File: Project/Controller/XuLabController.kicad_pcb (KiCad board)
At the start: 4 copper layers, 115 x 123 mm, 75 parts, among them J1 SWD Connector, J10 Servo, J11 Servo, J12 Thruster, J13 USB_B_Micro, J14 CAN, J15 I2C, J16 UART, J2 Conn_01x04, J3 1986660-2, J4 Servo, J5 Servo, J6 Servo, J7 Servo, J8 Servo, J9 Servo, Q2 PMOS, SW1 SW_Push, SW2 SW_SPDT, SW3 SW_SPDT, U1 STM32F446RCTx, U2 BMI088, U3 MMC5983MA, U4 AP63203WU, U5 TVS0500DRV, Y1 25 MHz

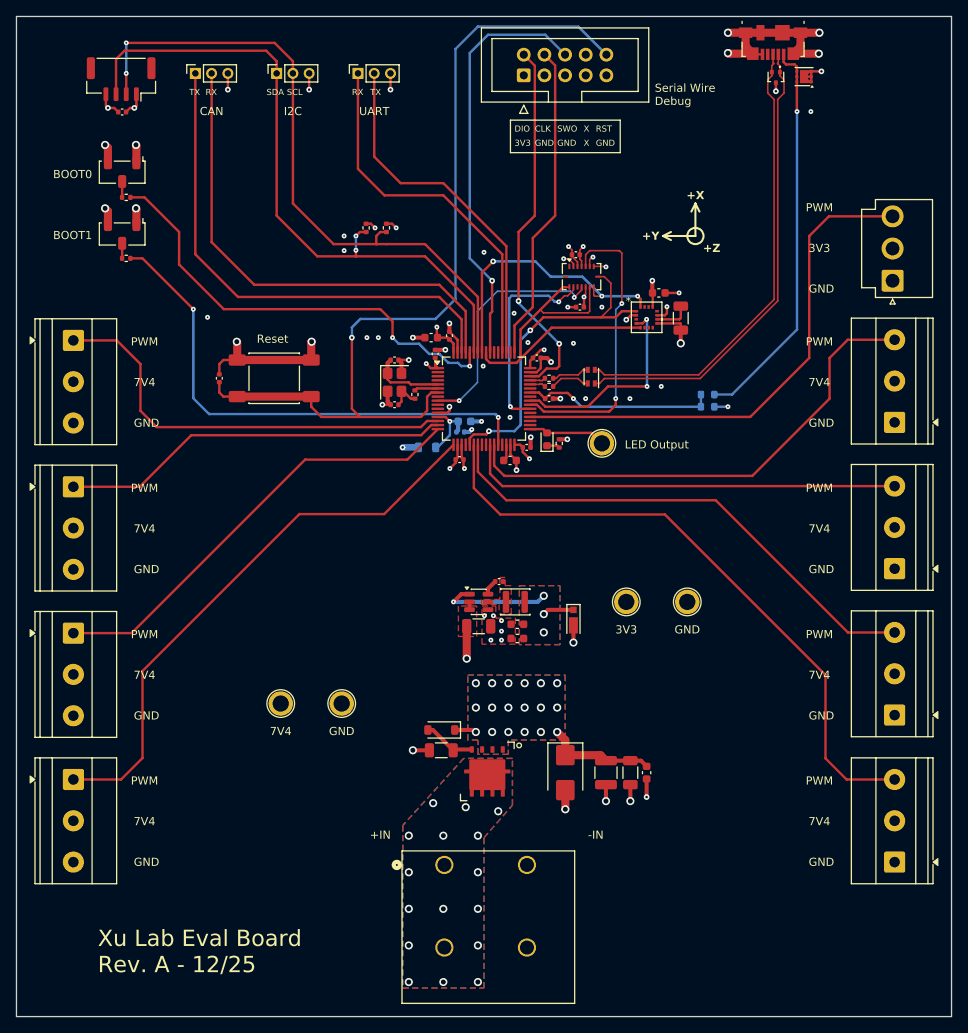
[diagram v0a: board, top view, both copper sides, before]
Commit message: Add initial layout
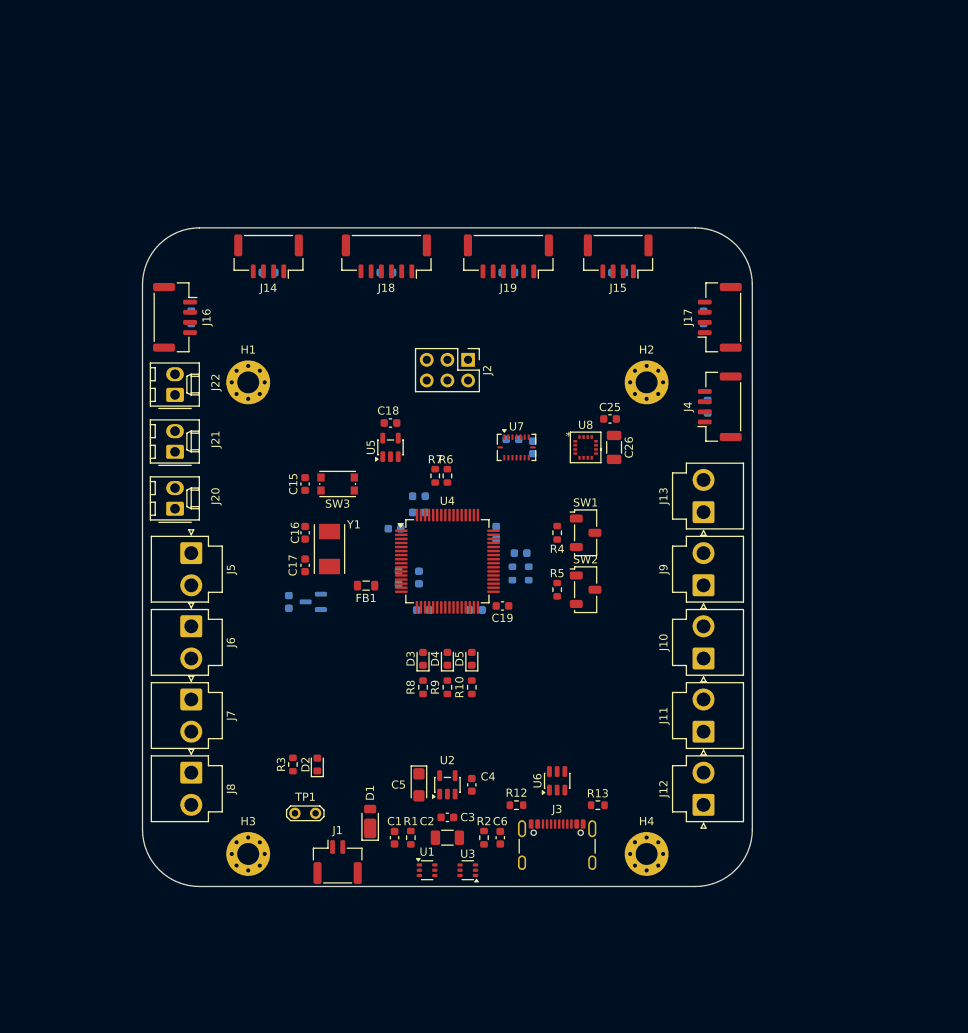
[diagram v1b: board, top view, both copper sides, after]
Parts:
- removed FL1: 0805USB-502MLC, Inductor_SMD:L_CommonModeChoke_Coilcraft_0805USB
- removed L1: 3.9uH, Inductor_SMD:L_Pulse_PA4334
- removed Q2: PMOS, XuLab:SOP-Advance-8
- removed TP2, TP3, TP4, TP5: TestPoint, TestPoint:TestPoint_Plated_Hole_D2.0mm
- added C26: 10uF, Capacitor_SMD:C_1206_3216Metric, F.Cu at (166.0, 86.0)
- added C27: 100nF, Capacitor_SMD:C_0603_1608Metric, B.Cu at (123.5, 64.5)
- added C28: 100nF, Capacitor_SMD:C_0603_1608Metric, B.Cu at (166.5, 64.5)
- added C29: 100nF, Capacitor_SMD:C_0603_1608Metric, B.Cu at (114.0, 70.0)
- added C30: 100nF, Capacitor_SMD:C_0603_1608Metric, B.Cu at (177.0, 70.0)
- added C31: 100nF, Capacitor_SMD:C_0603_1608Metric, B.Cu at (138.0, 64.5)
- added C32: 100nF, Capacitor_SMD:C_0603_1608Metric, B.Cu at (153.0, 64.5)
- added H1: MH, MountingHole:MountingHole_2.7mm_M2.5_Pad_Via, F.Cu at (121.0, 78.0)
- added H2: MH, MountingHole:MountingHole_2.7mm_M2.5_Pad_Via, F.Cu at (170.0, 78.0)
- added H3: MH, MountingHole:MountingHole_2.7mm_M2.5_Pad_Via, F.Cu at (121.0, 136.0)
- added H4: MH, MountingHole:MountingHole_2.7mm_M2.5_Pad_Via, F.Cu at (170.0, 136.0)
- added J17: UART2, Connector_JST:JST_GH_SM04B-GHS-TB_1x04-1MP_P1.25mm_Horizontal, F.Cu at (179.0, 70.0)
- added J18: SPI1, Connector_JST:JST_GH_SM06B-GHS-TB_1x06-1MP_P1.25mm_Horizontal, F.Cu at (138.0, 62.5)
- added J19: SPI2, Connector_JST:JST_GH_SM06B-GHS-TB_1x06-1MP_P1.25mm_Horizontal, F.Cu at (153.0, 62.5)
- added J20: Interrupt, Connector_Molex:Molex_KK-254_AE-6410-02A_1x02_P2.54mm_Vertical, F.Cu at (112.0, 93.5)
- added J21: Interrupt, Connector_Molex:Molex_KK-254_AE-6410-02A_1x02_P2.54mm_Vertical, F.Cu at (112.0, 86.5)
- added J22: Interrupt, Connector_Molex:Molex_KK-254_AE-6410-02A_1x02_P2.54mm_Vertical, F.Cu at (112.0, 79.5)
- added R12: 5k1, Resistor_SMD:R_0603_1608Metric, F.Cu at (154.0, 130.0)
- added R13: 5k1, Resistor_SMD:R_0603_1608Metric, F.Cu at (164.0, 130.0)
- added R14: 82k, Resistor_SMD:R_0603_1608Metric, B.Cu at (155.5, 101.5)
- added U6: USBLC6-2SC6, Package_TO_SOT_SMD:SOT-23-6, F.Cu at (159.0, 127.0)
- added U7: BMI088, Package_LGA:Bosch_LGA-16_4.5x3mm_P0.5mm_LayoutBorder7x1y_ClockwisePinNumbering, F.Cu at (154.0, 86.0)
- added U8: MMC5983MA, XuLab:MMC5983MA_MEM, F.Cu at (162.5, 86.0)
- added U9: MCP9700Ax-ETT, Package_TO_SOT_SMD:SOT-23, B.Cu at (129.0, 105.0)
- C1: value 4.7uF -> 1uF
- C10, C14, C22: footprint Capacitor_SMD:C_0402_1005Metric -> Capacitor_SMD:C_0603_1608Metric; moved to B.Cu
- C11, C12: value 22pF -> 100nF; footprint Capacitor_SMD:C_0402_1005Metric -> Capacitor_SMD:C_0603_1608Metric; moved to B.Cu
- C13: value 100nF -> 1uF; footprint Capacitor_SMD:C_0402_1005Metric -> Capacitor_SMD:C_0603_1608Metric; moved to B.Cu
- C15: value 1uF -> 100nF
- C16: value 10uF -> 27pF; footprint Capacitor_SMD:C_1206_3216Metric -> Capacitor_SMD:C_0603_1608Metric
- C17: value 100nF -> 27pF; footprint Capacitor_SMD:C_0402_1005Metric -> Capacitor_SMD:C_0603_1608Metric
- C18: value 100uF -> 100nF; footprint Capacitor_SMD:C_1210_3225Metric -> Capacitor_SMD:C_0603_1608Metric
- C19: value 10uF -> 2.2uF; footprint Capacitor_SMD:C_1206_3216Metric -> Capacitor_SMD:C_0603_1608Metric
- C2: value 100nF -> 10uF; footprint Capacitor_SMD:C_0402_1005Metric -> Capacitor_SMD:C_1206_3216Metric
- C20: value 1uF -> 100nF; moved to B.Cu
- C21: value 10uF -> 100nF; footprint Capacitor_SMD:C_1206_3216Metric -> Capacitor_SMD:C_0603_1608Metric; moved to B.Cu
- C23, C24: value 22uF -> 100nF; moved to B.Cu
- C25, C3, C6: value 100nF -> 1uF; footprint Capacitor_SMD:C_0402_1005Metric -> Capacitor_SMD:C_0603_1608Metric
- C4: value 100nF -> 470pF; footprint Capacitor_SMD:C_0402_1005Metric -> Capacitor_SMD:C_0603_1608Metric
- C5: value 100nF -> 2.2uF; footprint Capacitor_SMD:C_0402_1005Metric -> Capacitor_Tantalum_SMD:CP_EIA-3216-18_Kemet-A
- C7: value 1uF -> 4.7uF
- C8: footprint Capacitor_SMD:C_0402_1005Metric -> Capacitor_SMD:C_0603_1608Metric
- C9: value 2.2uF -> 100nF; moved to B.Cu
- D1: value LED -> 5V; footprint LED_SMD:LED_0603_1608Metric -> Diode_SMD:D_PowerDI-123
- D2: value RCLAMP0582B -> Red; footprint Package_TO_SOT_SMD:SOT-416 -> LED_SMD:LED_0603_1608Metric
- D3: value 12V -> Amber; footprint Diode_SMD:D_SOD-123 -> LED_SMD:LED_0603_1608Metric
- D4: value 7.5V -> Green; footprint Diode_SMD:D_SMB -> LED_SMD:LED_0603_1608Metric
- D5: value 3.3V -> Blue; footprint Diode_SMD:D_MicroSMP_KA -> LED_SMD:LED_0603_1608Metric
- FB1: moved to F.Cu
- J1: value SWD Connector -> Power; footprint Connector_IDC:IDC-Header_2x05_P2.54mm_Vertical -> Connector_JST:JST_GH_SM02B-GHS-TB_1x02-1MP_P1.25mm_Horizontal
- J10, J11, J5, J6, J7, J8, J9: footprint TerminalBlock_Phoenix:TerminalBlock_Phoenix_MKDS-1,5-3-5.08_1x03_P5.08mm_Horizontal -> Connector_JST:JST_VH_B2P-VH_1x02_P3.96mm_Vertical
- J12: value Thruster -> Servo; footprint Connector_JST:JST_VH_B3P-VH_1x03_P3.96mm_Vertical -> Connector_JST:JST_VH_B2P-VH_1x02_P3.96mm_Vertical
- J13: value USB_B_Micro -> Thruster; footprint Connector_USB:USB_Micro-B_Molex_47346-0001 -> Connector_JST:JST_VH_B2P-VH_1x02_P3.96mm_Vertical
- J14: value CAN -> I2C; footprint Connector_PinSocket_2.00mm:PinSocket_1x03_P2.00mm_Vertical -> Connector_JST:JST_GH_SM04B-GHS-TB_1x04-1MP_P1.25mm_Horizontal
- J15: footprint Connector_PinSocket_2.00mm:PinSocket_1x03_P2.00mm_Vertical -> Connector_JST:JST_GH_SM04B-GHS-TB_1x04-1MP_P1.25mm_Horizontal
- J16: value UART -> UART1; footprint Connector_PinSocket_2.00mm:PinSocket_1x03_P2.00mm_Vertical -> Connector_JST:JST_GH_SM04B-GHS-TB_1x04-1MP_P1.25mm_Horizontal
- J2: value Conn_01x04 -> SWD; footprint Connector_JST:JST_GH_SM04B-GHS-TB_1x04-1MP_P1.25mm_Horizontal -> Connector_PinHeader_2.54mm:PinHeader_2x03_P2.54mm_Vertical
- J3: value 1986660-2 -> USB_C_Receptacle_USB2.0_16P; footprint XuLab:CONN2_1986660-2_TEC -> Connector_USB:USB_C_Receptacle_GCT_USB4105-xx-A_16P_TopMnt_Horizontal
- J4: value Servo -> Bar30; footprint TerminalBlock_Phoenix:TerminalBlock_Phoenix_MKDS-1,5-3-5.08_1x03_P5.08mm_Horizontal -> Connector_JST:JST_GH_SM04B-GHS-TB_1x04-1MP_P1.25mm_Horizontal
- R1, R2: value 10k -> 47k; footprint Resistor_SMD:R_0402_1005Metric -> Resistor_SMD:R_0603_1608Metric
- R10: value 10k -> 100; moved to F.Cu
- R11: value 20k -> 33k
- R3: value 270 -> 330; footprint Resistor_SMD:R_0402_1005Metric -> Resistor_SMD:R_0603_1608Metric
- R4, R5: value 4k7 -> 10k; footprint Resistor_SMD:R_0402_1005Metric -> Resistor_SMD:R_0603_1608Metric
- R6, R7: value 22 -> 4k7; footprint Resistor_SMD:R_0402_1005Metric -> Resistor_SMD:R_0603_1608Metric
- R8: value 75 -> 330; footprint Resistor_SMD:R_0402_1005Metric -> Resistor_SMD:R_0603_1608Metric
- R9: value 100 -> 330; footprint Resistor_SMD:R_1206_3216Metric -> Resistor_SMD:R_0603_1608Metric
- SW1: value SW_Push -> SW_SPDT; footprint Button_Switch_SMD:SW_Push_1P1T_NO_E-Switch_TL3301NxxxxxG -> Button_Switch_SMD:Nidec_Copal_CAS-120A
- SW3: value SW_SPDT -> SW_Push; footprint Button_Switch_SMD:Nidec_Copal_CAS-120A -> Button_Switch_SMD:SW_Push_1P1T_NO_CK_KMR2
- TP1: value TestPoint -> Power; footprint TestPoint:TestPoint_Plated_Hole_D2.0mm -> TestPoint:TestPoint_2Pads_Pitch2.54mm_Drill0.8mm
- U1: value STM32F446RCTx -> LM66100DCK; footprint Package_QFP:LQFP-64_10x10mm_P0.5mm -> Package_TO_SOT_SMD:SOT-363_SC-70-6
- U2: value BMI088 -> MIC5219-3.3YM5; footprint Package_LGA:Bosch_LGA-16_4.5x3mm_P0.5mm_LayoutBorder7x1y_ClockwisePinNumbering -> Package_TO_SOT_SMD:SOT-23-5
- U3: value MMC5983MA -> LM66100DCK; footprint XuLab:MMC5983MA_MEM -> Package_TO_SOT_SMD:SOT-363_SC-70-6
- U4: value AP63203WU -> STM32F446RCTx; footprint Package_TO_SOT_SMD:TSOT-23-6 -> Package_QFP:LQFP-64_10x10mm_P0.5mm
- U5: value TVS0500DRV -> 24AA64-OT; footprint Package_SON:WSON-6-1EP_2x2mm_P0.65mm_EP1x1.6mm -> Package_TO_SOT_SMD:SOT-23-5
- Y1: value 25 MHz -> 8MHz; footprint Crystal:Crystal_SMD_Abracon_ABM8G-4Pin_3.2x2.5mm -> Crystal:Crystal_SMD_Abracon_ABM7-2Pin_6.0x3.5mm
- moved D2 101.6 mm to (129.5, 125.0), turned to 90 degrees
- moved J1 99.4 mm to (132.0, 137.0), turned to 0 degrees
- moved J8 87.2 mm to (114.0, 126.0), turned to -90 degrees
- moved R1 86.2 mm to (141.0, 134.0), turned to -90 degrees
- moved R2 83.7 mm to (150.0, 134.0), turned to 90 degrees
- moved J4 79.9 mm to (179.0, 81.0), turned to 90 degrees
- moved SW2 76.7 mm to (162.5, 103.5), turned to 0 degrees
- moved U3 71.5 mm to (148.0, 138.0), turned to 180 degrees
- moved J12 68.5 mm to (177.0, 130.0)
- moved U5 68.3 mm to (138.5, 86.0), turned to 90 degrees
- moved U2 64.6 mm to (145.5, 127.5), turned to 90 degrees
- moved C1 61.7 mm to (139.0, 134.0), turned to -90 degrees
- moved C17 60.1 mm to (128.0, 100.5), turned to 90 degrees
- moved C2 59.5 mm to (145.5, 134.0), turned to 0 degrees
- moved C3 59.3 mm to (145.5, 131.5), turned to 0 degrees
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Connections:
- C1 pad 1: +3.3V -> Net-(D1-K)
- C10 pad 1: /MCU A/NRST -> +3.3V
- C11 pad 1: /MCU A/RCC_IN -> +3.3V
- C12 pad 1: Net-(C12-Pad1) -> +3.3V
- C13 pad 1: +3.3V -> +3.3VA
- C14 pad 1: +3.3V -> +3.3VA
- C15 pad 1: +3.3V -> /Microcontroller/NRST
- C16 pad 1: Net-(U3-CAP) -> /Microcontroller/RCC_IN
- C17 pad 1: +3.3V -> /Microcontroller/RCC_OUT
- C18 pad 1: +7.4V -> +3.3V
- C19 pad 1: +7.4V -> Net-(U4-VCAP_1)
- C2 pad 1: +3.3V -> Net-(U1-VOUT)
- C20 pad 1: +7.4V -> /Microcontroller/USB_VBUS
- C21 pad 1: +7.4V -> +3.3V
- C22 pad 1: Net-(U4-BST) -> +3.3V
- C22 pad 2: Net-(U4-SW) -> GND
- C25 pad 1: /MCU A/USB_VBUS -> +3.3V
- C3 pad 1: +3.3V -> Net-(U1-VOUT)
- C4 pad 1: +3.3V -> Net-(U2-BP)
- C6 pad 1: +3.3V -> /USB_Power
- C7 pad 1: +3.3VA -> +3.3V
- C8 pad 1: +3.3VA -> +3.3V
- C9 pad 1: Net-(U1-VCAP_1) -> +3.3V
- D1 pad 2: /MCU A/LED_OUT -> GND
- D2 pad 1: /MCU A/USB_D_I- -> Net-(D2-K)
- D2 pad 2: /MCU A/USB_D_I+ -> +3.3V
- D3 pad 1: +7.4V -> Net-(D3-K)
- D3 pad 2: Net-(D3-A) -> /Microcontroller/LED_OUT1
- D4 pad 1: +7.4V -> Net-(D4-K)
- D4 pad 2: GND -> /Microcontroller/LED_OUT2
- D5 pad 1: +3.3V -> Net-(D5-K)
- D5 pad 2: GND -> /Microcontroller/LED_OUT3
- J1 pad 1: +3.3V -> Net-(D1-K)
- J1 pad 2: /MCU A/SW_DIO -> GND
- J10 pad 1: GND -> /PWM_6
- J10 pad 2: +7.4V -> GND
- J11 pad 1: GND -> /PWM_7
- J11 pad 2: +7.4V -> GND
- J12 pad 1: GND -> /PWM_8
- J12 pad 2: +3.3V -> GND
- J13 pad 1: /MCU A/USB_VBUS_I -> /PWM_9
- J13 pad 2: /MCU A/USB_D_I- -> GND
- J14 pad 1: /CAN1_TX -> +3.3V
- J14 pad 2: /CAN1_RX -> /I2C1_SCL
- J14 pad 3: GND -> /I2C1_SDA
- J15 pad 1: /I2C1_SDA -> +3.3V
- J15 pad 3: GND -> /I2C1_SDA
- J16 pad 1: /UART_RX -> +3.3V
- J16 pad 2: /UART_TX -> /UART1_TX
- J16 pad 3: GND -> /UART1_RX
- J2 pad 2: /I2C1_SCL -> /Microcontroller/SW_DIO
- J2 pad 3: /I2C1_SDA -> /Microcontroller/NRST
- J2 pad 4: GND -> /Microcontroller/SW_CLK
- J4 pad 1: /PWM_1 -> +3.3V
- J4 pad 2: +7.4V -> /I2C1_SCL
- J4 pad 3: GND -> /I2C1_SDA
- J5 pad 1: /PWM_2 -> /PWM_1
- J5 pad 2: +7.4V -> GND
- J6 pad 1: /PWM_3 -> /PWM_2
- J6 pad 2: +7.4V -> GND
- J7 pad 1: /PWM_4 -> /PWM_3
- J7 pad 2: +7.4V -> GND
- J8 pad 1: GND -> /PWM_4
- J8 pad 2: +7.4V -> GND
- J9 pad 1: GND -> /PWM_5
- J9 pad 2: +7.4V -> GND
- R1 pad 1: Net-(SW2-B) -> Net-(D1-K)
- R1 pad 2: /MCU A/BOOT0 -> /Power/Status
- R10 pad 1: /MCU A/USB_VBUS_I -> Net-(D5-K)
- R10 pad 2: /MCU A/USB_VBUS -> GND
- R11 pad 1: /MCU A/USB_VBUS -> /USB_Power
- R11 pad 2: GND -> /Microcontroller/USB_VBUS
- R2 pad 1: Net-(SW3-B) -> Net-(U1-~{CE})
- R2 pad 2: /MCU A/BOOT1 -> /USB_Power
- R3 pad 1: /MCU A/RCC_OUT -> Net-(D2-K)
- R3 pad 2: Net-(C12-Pad1) -> GND
- R4 pad 1: +3.3V -> Net-(SW1-B)
- R4 pad 2: /I2C1_SCL -> /Microcontroller/BOOT0
- R5 pad 1: +3.3V -> Net-(SW2-B)
- R5 pad 2: /I2C1_SDA -> /Microcontroller/BOOT1
- R6 pad 1: /MCU A/USB_D+ -> +3.3V
- R6 pad 2: /MCU A/USB_D_M+ -> /I2C1_SCL
- R7 pad 1: /MCU A/USB_D- -> +3.3V
- R7 pad 2: /MCU A/USB_D_M- -> /I2C1_SDA
- R8 pad 1: Net-(D1-K) -> Net-(D3-K)
- R9 pad 1: Net-(D3-A) -> Net-(D4-K)
- SW1 pad 1: /MCU A/NRST -> GND
- SW1 pad 2: GND -> Net-(SW1-B)
- SW3 pad 1: GND -> /Microcontroller/NRST
- SW3 pad 2: Net-(SW3-B) -> GND
- TP1 pad 1: +7.4V -> +3.3V
- U1 pad 1: +3.3V -> Net-(D1-K)
- U1 pad 2: unconnected-(U1-PC13-Pad2) -> GND
- U1 pad 3: unconnected-(U1-PC14-Pad3) -> Net-(U1-~{CE})
- U1 pad 5: /MCU A/RCC_IN -> /Power/Status
- U1 pad 6: /MCU A/RCC_OUT -> Net-(U1-VOUT)
- U2 pad 1: /Attitude and Heading Module/ACCL_INT2 -> Net-(U1-VOUT)
- U2 pad 3: +3.3V -> Net-(U1-VOUT)
- U2 pad 4: GND -> Net-(U2-BP)
- U2 pad 5: /SPI1_CS2 -> +3.3V
- U3 pad 1: /SPI1_SCK -> /USB_Power
- U3 pad 2: +3.3V -> GND
- U3 pad 3: unconnected-(U3-NC-Pad3) -> /Power/Status
- U3 pad 4: /SPI1_CS3 -> unconnected-(U3-NC-Pad4)
- U3 pad 5: /SPI1_MISO -> unconnected-(U3-ST-Pad5)
- U3 pad 6: unconnected-(U3-NC-Pad6) -> Net-(U1-VOUT)
- U4 pad 2: +7.4V -> /GPIO_EXTI13
- U4 pad 3: +7.4V -> /GPIO_EXTI14
- U4 pad 4: GND -> /GPIO_EXTI15
- U4 pad 5: Net-(U4-SW) -> /Microcontroller/RCC_IN
- U4 pad 6: Net-(U4-BST) -> /Microcontroller/RCC_OUT
- U5 pad 1: GND -> /I2C1_SCL
- U5 pad 3: GND -> /I2C1_SDA
- U5 pad 4: /MCU A/USB_VBUS_I -> +3.3V
- U5 pad 5: /MCU A/USB_VBUS_I -> GND
- Y1 pad 1: /MCU A/RCC_IN -> /Microcontroller/RCC_IN
- Y1 pad 2: GND -> /Microcontroller/RCC_OUT
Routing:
- net GND: track 127.6 -> 0.00 mm, vias 65 -> 0
- net /MCU A/NRST: track 109.9 -> 0.00 mm, vias 1 -> 0
- net /I2C1_SDA: track 82.6 -> 0.00 mm, vias 2 -> 0
- net /I2C1_SCL: track 82.0 -> 0.00 mm, vias 2 -> 0
- net /PWM_5: track 77.9 -> 0.00 mm
- net /PWM_4: track 70.1 -> 0.00 mm
- net /PWM_9: track 63.6 -> 0.00 mm
- net /MCU A/BOOT1: track 63.2 -> 0.00 mm, vias 2 -> 0
- net /PWM_6: track 62.8 -> 0.00 mm
- net /CAN1_TX: track 62.4 -> 0.00 mm
- net /PWM_8: track 62.2 -> 0.00 mm
- net /CAN1_RX: track 60.6 -> 0.00 mm
- net /MCU A/USB_D_I-: track 57.7 -> 0.00 mm
- net +3.3V: track 57.0 -> 0.00 mm, vias 19 -> 0
- net /MCU A/USB_D_I+: track 57.0 -> 0.00 mm
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- removed copper zone on B.Cu, net +3.3V
- removed copper zone on F.Cu, net +3.3V
- removed copper zone on In2.Cu, net +3.3V
- removed copper zone on B.Cu, net +7.4V
- removed copper zone on F.Cu, net +7.4V
- removed copper zone on In2.Cu, net +7.4V
- removed copper zone on F.Cu, net GND
- removed copper zone on In1.Cu, net GND
- removed copper zone on B.Cu, net Net-(Q2-D)
- removed copper zone on F.Cu, net Net-(Q2-D)
- removed copper zone on F.Cu, net Net-(U4-SW)
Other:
- board size 115 x 123 mm -> 75 x 81 mm
- board text removed: "+IN"
- board text removed: "+X"
- board text removed: "+Y"
- board text removed: "+Z"
- board text removed: "-IN"
- board text removed: "3V3"
- board text removed: "7V4"
- board text removed: "BOOT0"
- board text removed: "BOOT1"
- board text removed: "CAN"
- board text removed: "CLK"
- board text removed: "DIO"
- board text removed: "GND"
- board text removed: "I2C"
- board text removed: "LED Output"
- board text removed: "PWM"
- board text removed: "RST"
- board text removed: "RX"
- board text removed: "Reset"
- board text removed: "SCL"
- board text removed: "SDA"
- board text removed: "SWO"
- board text removed: "Serial Wire Debug"
- board text removed: "TX"
- board text removed: "UART"
- board text removed: "X"
- board text removed: "Xu Lab Eval Board Rev. A - 12/25"
